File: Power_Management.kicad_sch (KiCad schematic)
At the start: 17 parts, among them J8 PWR_SRC_JMP, Q1 MOSFET_SI2333DDS-T1-BE3, U3 SN74LVC1G07DBVR

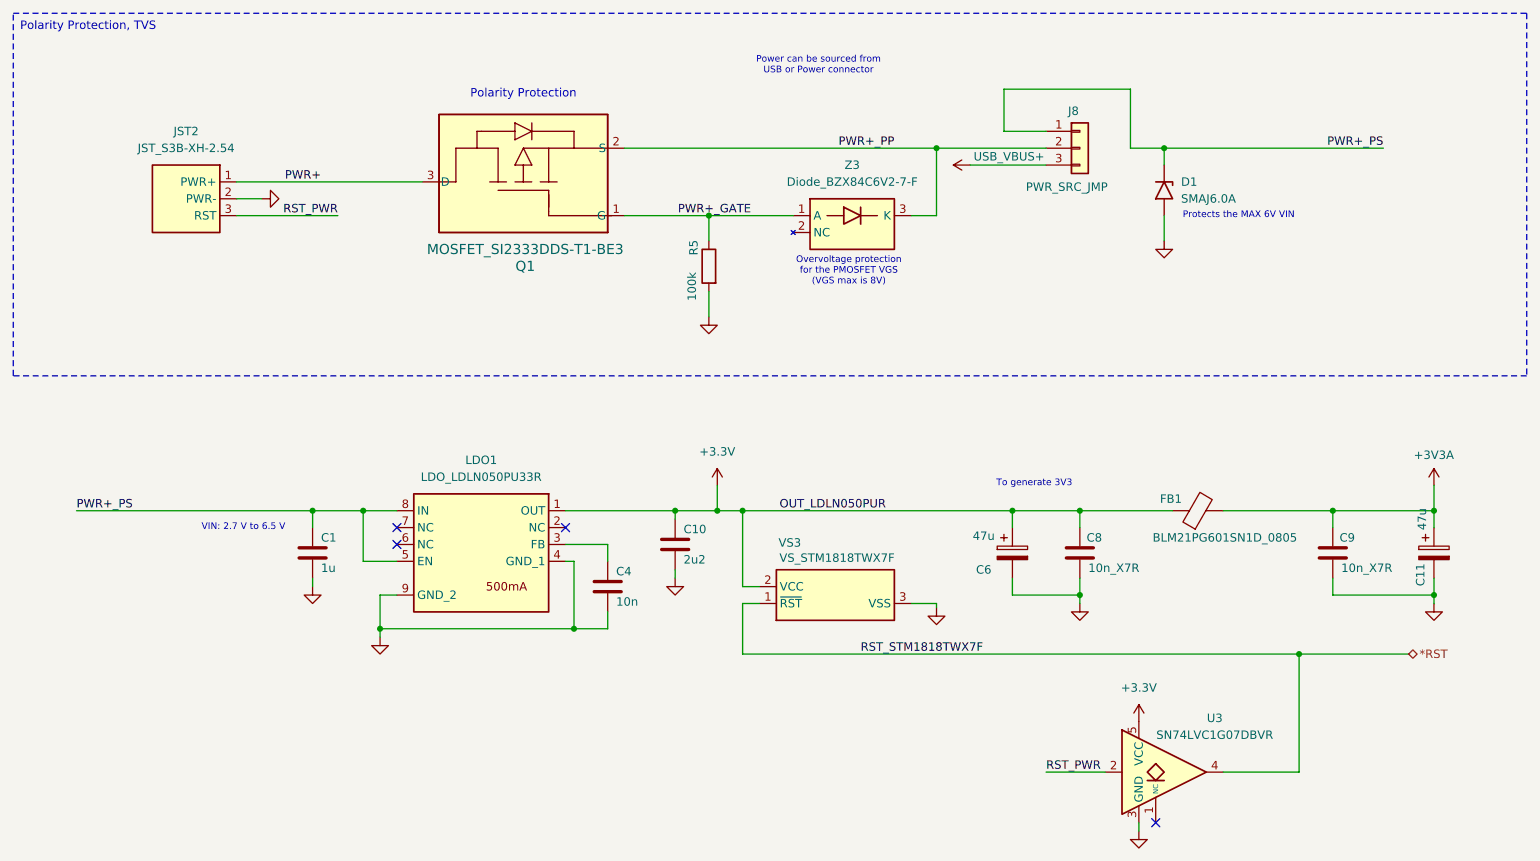
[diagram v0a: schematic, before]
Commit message: Update
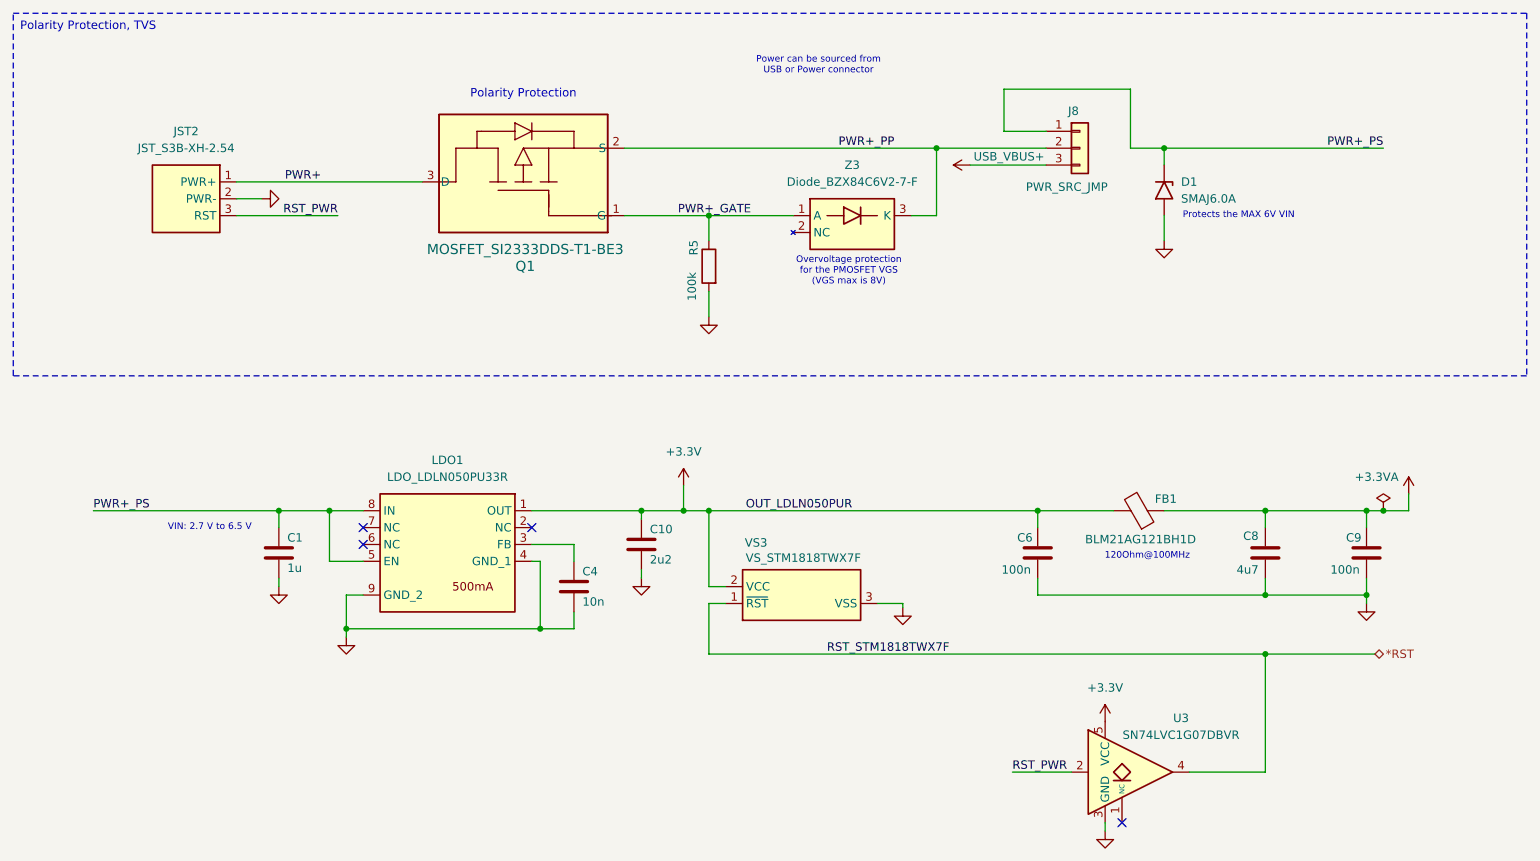
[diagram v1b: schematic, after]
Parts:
- removed C11, C6: 47u, Capacitor_SMD:C_0805_2012Metric, symbol Device:C_Polarized
- added C6: 100n, Capacitor_SMD:C_0805_2012Metric, symbol Device:C
- C8: value 10n_X7R -> 4u7
- C9: value 10n_X7R -> 100n
- FB1: value BLM21PG601SN1D_0805 -> BLM21AG121BH1D
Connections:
- net +3.3V: now also FB1.2, C6.1; no longer C8.1, FB1.1
- net GND: now also C6.2
- net +3V3A renamed +3.3VA
- net +3.3VA: now also C8.1, FB1.1; no longer FB1.2
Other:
- note added: "120Ohm@100MHz"
- note removed: "To generate 3V3"
- moved on the sheet: C1, C10, C4, LDO1, U3, VS3
